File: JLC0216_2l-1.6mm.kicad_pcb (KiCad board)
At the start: 4 copper layers, 24 x 24 mm, 0 parts

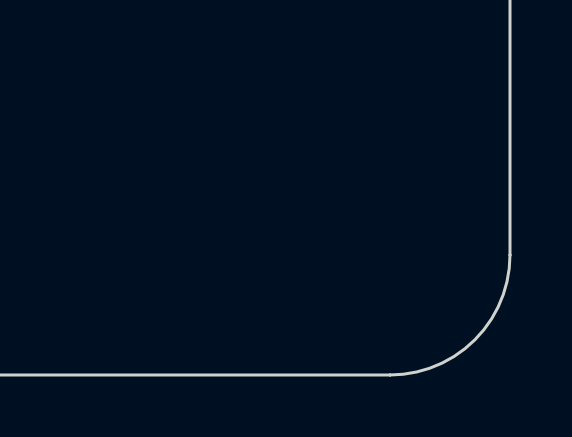
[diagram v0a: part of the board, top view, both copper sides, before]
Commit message: update stack
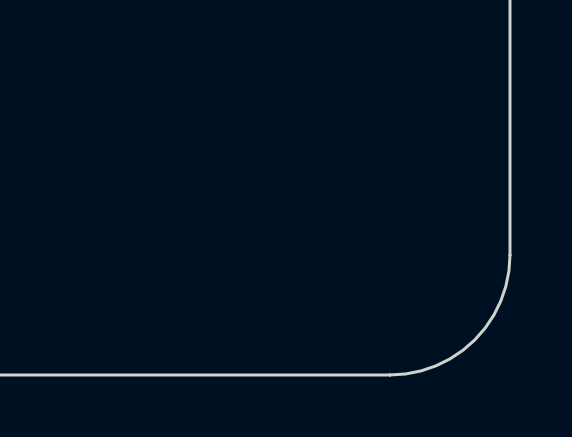
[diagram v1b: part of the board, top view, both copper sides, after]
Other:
- copper layers 4 -> 2
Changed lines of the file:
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@@
 	(generator_version "8.0")
 	(general
-		(thickness 1.5742)
+		(thickness 1.555)
 		(legacy_teardrops no)
 	)
@@
 		(date "SET!!!")
 		(rev "VERV")
-		(company "ELT")
+		(company "SET!!!")
 		(comment 2 "SET!!!")
 		(comment 3 "SET!!!")
@@
 	(layers
 		(0 "F.Cu" signal)
-		(1 "In1.Cu" power)
-		(2 "In2.Cu" power)
 		(31 "B.Cu" signal)
 		(32 "B.Adhes" user "B.Adhesive")
@@
 			(layer "F.Mask"
 				(type "Top Solder Mask")
-				(thickness 0.005)
+				(thickness 0.01)
 			)
 			(layer "F.Cu"
@@
 			)
 			(layer "dielectric 1"
-				(type "prepreg")
-				(thickness 0.0994)
-				(material "3313")
-				(epsilon_r 4.1)
-				(loss_tangent 0.002)
-			)
-			(layer "In1.Cu"
-				(type "copper")
-				(thickness 0.0152)
-			)
-			(layer "dielectric 2"
 				(type "core")
 				(color "FR4 natural")
-				(thickness 1.265)
+				(thickness 1.465)
 				(material "FR4")
 				(epsilon_r 4.5)
 				(loss_tangent 0.02)
 			)
-			(layer "In2.Cu"
-				(type "copper")
-				(thickness 0.0152)
-			)
-			(layer "dielectric 3"
-				(type "prepreg")
-				(color "FR4 natural")
-				(thickness 0.0994)
-				(material "3313")
-				(epsilon_r 4.1)
-				(loss_tangent 0.002)
-			)
 			(layer "B.Cu"
 				(type "copper")
@@
 			(layer "B.Mask"
 				(type "Bottom Solder Mask")
-				(thickness 0.005)
+				(thickness 0.01)
 			)
 			(layer "B.Paste"
@@
 			)
 			(copper_finish "HAL SnPb")
-			(dielectric_constraints no)
+			(dielectric_constraints yes)
 		)
 		(pad_to_mask_clearance 0)
@@
 		(layer "Dwgs.User")
 	)
+	(gr_line
+		(start 34 30)
+		(end 50 30)
+		(stroke
+			(width 0.1)
+			(type default)
+		)
+		(layer "Edge.Cuts")
+	)
+	(gr_arc
+		(start 54 50)
+		(mid 52.828427 52.828427)
+		(end 49.999999 54.000001)
+		(stroke
+			(width 0.1)
+			(type default)
+		)
+		(layer "Edge.Cuts")
+	)
+	(gr_line
+		(start 49.999999 54.000001)
+		(end 33.999999 54.000001)
+		(stroke
+			(width 0.1)
+			(type default)
+		)
+		(layer "Edge.Cuts")
+	)
+	(gr_arc
+		(start 29.999999 34.000001)
+		(mid 31.171572 31.171573)
+		(end 34 30)
+		(stroke
+			(width 0.1)
+			(type default)
+		)
+		(layer "Edge.Cuts")
+	)
+	(gr_arc
+		(start 50 30)
+		(mid 52.828428 31.171573)
+		(end 54.000001 34.000001)
+		(stroke
+			(width 0.1)
+			(type default)
+		)
+		(layer "Edge.Cuts")
+	)
+	(gr_line
+		(start 29.999999 34.000001)
+		(end 29.999999 50)
+		(stroke
+			(width 0.1)
+			(type default)
+		)
+		(layer "Edge.Cuts")
+	)
 	(gr_arc
 		(start 34.000001 54.000001)
@@
 		(layer "Edge.Cuts")
 	)
-	(gr_arc
-		(start 50 30)
-		(mid 52.828428 31.171573)
-		(end 54.000001 34.000001)
-		(stroke
-			(width 0.1)
-			(type default)
-		)
-		(layer "Edge.Cuts")
-	)
-	(gr_line
-		(start 34 30)
-		(end 50 30)
-		(stroke
-			(width 0.1)
-			(type default)
-		)
-		(layer "Edge.Cuts")
-	)
-	(gr_arc
-		(start 54 50)
-		(mid 52.828427 52.828428)
-		(end 49.999999 54.000001)
-		(stroke
-			(width 0.1)
-			(type default)
-		)
-		(layer "Edge.Cuts")
-	)
 	(gr_line
 		(start 54 49.999999)
@@
 		(stroke
 			(width 0.1)
-			(type default)
-		)
-		(layer "Edge.Cuts")
-	)
-	(gr_line
-		(start 49.999999 54.000001)
-		(end 33.999999 54.000001)
-		(stroke
-			(width 0.1)
-			(type default)
-		)
-		(layer "Edge.Cuts")
-	)
-	(gr_arc
-		(start 29.999999 34.000001)
-		(mid 31.171572 31.171573)
-		(end 34 30)
-		(stroke
-			(width 0.1)
-			(type default)
-		)
-		(layer "Edge.Cuts")
-	)
-	(gr_line
-		(start 29.999999 34.000001)
-		(end 29.999999 50)
-		(stroke
-			(width 0.1)
